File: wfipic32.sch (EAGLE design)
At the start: 31 parts, among them IC1 BMA490L, J1 MLE-105-01-G-DV, J2 MLE-105-01-G-DV, J3 MLE-105-01-G-DV, J4 MLE-105-01-G-DV, U1 PIC32MK0512MCJ048T-I/Y8XTQFP4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, U2 MAX6126B30

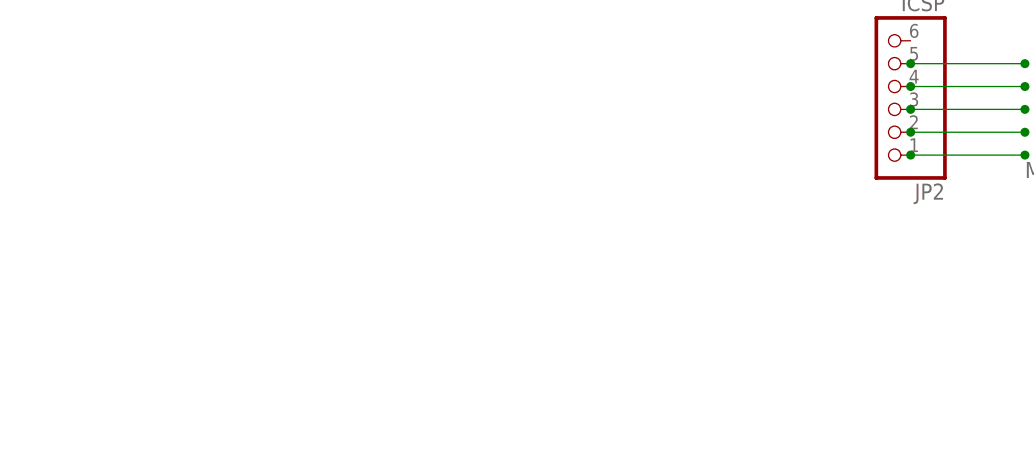
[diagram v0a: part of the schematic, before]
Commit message: up
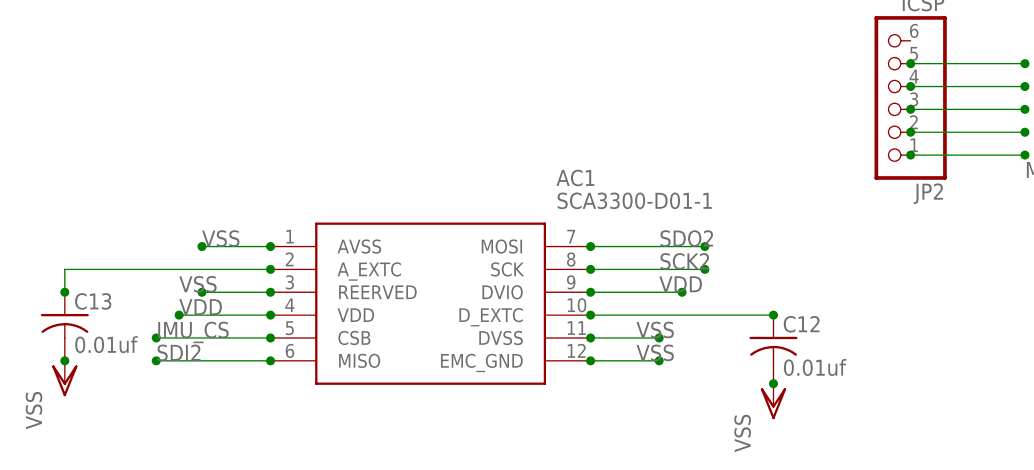
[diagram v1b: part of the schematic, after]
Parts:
- added AC1: SCA3300-D01-1, SCA3300-D01-1:SCA3300-D01-1
- added C12, C13: 0.01uf, rcl:C-USC0805
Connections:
- new net N$7: AC1.D_EXTC, C12.1
- new net N$9: AC1.A_EXTC, C13.1
- net IMU_CS: now also AC1.CSB
- net SCK2: now also AC1.SCK
- net SDI2: now also AC1.MISO
- net SDO2: now also AC1.MOSI
- net VDD: now also AC1.DVIO, AC1.VDD
- net VSS: now also AC1.AVSS, AC1.DVSS, AC1.EMC_GND, AC1.REERVED, C12.2, C13.2
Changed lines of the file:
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@@
 <part name="J4" library="MLE-105-01-G-DV" deviceset="MLE-105-01-G-DV" device=""/>
 <part name="VSS9" library="supply1" library_urn="urn:adsk.eagle:library:371" deviceset="VSS" device=""/>
+<part name="AC1" library="SCA3300-D01-1" deviceset="SCA3300-D01-1" device=""/>
+<part name="C12" library="rcl" library_urn="urn:adsk.eagle:library:334" deviceset="C-US" device="C0805" package3d_urn="urn:adsk.eagle:package:23617/2" value="0.01uf"/>
+<part name="C13" library="rcl" library_urn="urn:adsk.eagle:library:334" deviceset="C-US" device="C0805" package3d_urn="urn:adsk.eagle:package:23617/2" value="0.01uf"/>
+<part name="VSS21" library="supply1" library_urn="urn:adsk.eagle:library:371" deviceset="VSS" device=""/>
+<part name="VSS22" library="supply1" library_urn="urn:adsk.eagle:library:371" deviceset="VSS" device=""/>
 </parts>
 <sheets>
@@
 <instance part="VSS9" gate="G$1" x="93.98" y="139.7" smashed="yes" rot="R270">
 <attribute name="VALUE" x="88.9" y="142.24" size="1.778" layer="96"/>
+</instance>
+<instance part="AC1" gate="G$1" x="-30.48" y="-22.86" smashed="yes">
+<attribute name="NAME" x="1.27" y="-15.24" size="1.778" layer="95" align="center-left"/>
+<attribute name="VALUE" x="1.27" y="-17.78" size="1.778" layer="96" align="center-left"/>
+</instance>
+<instance part="C12" gate="G$1" x="25.4" y="-33.02" smashed="yes">
+<attribute name="NAME" x="26.416" y="-32.385" size="1.778" layer="95"/>
+<attribute name="VALUE" x="26.416" y="-37.211" size="1.778" layer="96"/>
+</instance>
+<instance part="C13" gate="G$1" x="-53.34" y="-30.48" smashed="yes">
+<attribute name="NAME" x="-52.324" y="-29.845" size="1.778" layer="95"/>
+<attribute name="VALUE" x="-52.324" y="-34.671" size="1.778" layer="96"/>
+</instance>
+<instance part="VSS21" gate="G$1" x="25.4" y="-40.64" smashed="yes">
+<attribute name="VALUE" x="22.86" y="-45.72" size="1.778" layer="96" rot="R90"/>
+</instance>
+<instance part="VSS22" gate="G$1" x="-53.34" y="-38.1" smashed="yes">
+<attribute name="VALUE" x="-55.88" y="-43.18" size="1.778" layer="96" rot="R90"/>
 </instance>
 </instances>
@@
 <junction x="132.08" y="144.78"/>
 </segment>
+<segment>
+<wire x1="-30.48" y1="-30.48" x2="-40.64" y2="-30.48" width="0.1524" layer="91"/>
+<pinref part="AC1" gate="G$1" pin="VDD"/>
+<label x="-40.64" y="-30.48" size="1.778" layer="95"/>
+<junction x="-30.48" y="-30.48"/>
+<junction x="-40.64" y="-30.48"/>
+</segment>
+<segment>
+<wire x1="15.24" y1="-27.94" x2="5.08" y2="-27.94" width="0.1524" layer="91"/>
+<pinref part="AC1" gate="G$1" pin="DVIO"/>
+<label x="12.7" y="-27.94" size="1.778" layer="95"/>
+<junction x="5.08" y="-27.94"/>
+<junction x="15.24" y="-27.94"/>
+</segment>
 </net>
 <net name="VSS" class="0">
@@
 <junction x="96.52" y="139.7"/>
 </segment>
+<segment>
+<wire x1="-30.48" y1="-22.86" x2="-38.1" y2="-22.86" width="0.1524" layer="91"/>
+<pinref part="AC1" gate="G$1" pin="AVSS"/>
+<label x="-38.1" y="-22.86" size="1.778" layer="95"/>
+<junction x="-30.48" y="-22.86"/>
+<junction x="-38.1" y="-22.86"/>
+</segment>
+<segment>
+<wire x1="12.7" y1="-33.02" x2="5.08" y2="-33.02" width="0.1524" layer="91"/>
+<pinref part="AC1" gate="G$1" pin="DVSS"/>
+<label x="10.16" y="-33.02" size="1.778" layer="95"/>
+<junction x="5.08" y="-33.02"/>
+<junction x="12.7" y="-33.02"/>
+</segment>
+<segment>
+<wire x1="12.7" y1="-35.56" x2="5.08" y2="-35.56" width="0.1524" layer="91"/>
+<pinref part="AC1" gate="G$1" pin="EMC_GND"/>
+<label x="10.16" y="-35.56" size="1.778" layer="95"/>
+<junction x="5.08" y="-35.56"/>
+<junction x="12.7" y="-35.56"/>
+</segment>
+<segment>
+<pinref part="C12" gate="G$1" pin="2"/>
+<pinref part="VSS21" gate="G$1" pin="VSS"/>
+<junction x="25.4" y="-38.1"/>
+</segment>
+<segment>
+<pinref part="C13" gate="G$1" pin="2"/>
+<pinref part="VSS22" gate="G$1" pin="VSS"/>
+<junction x="-53.34" y="-35.56"/>
+</segment>
+<segment>
+<wire x1="-30.48" y1="-27.94" x2="-38.1" y2="-27.94" width="0.1524" layer="91"/>
+<pinref part="AC1" gate="G$1" pin="REERVED"/>
+<label x="-40.64" y="-27.94" size="1.778" layer="95"/>
+<junction x="-38.1" y="-27.94"/>
+<junction x="-30.48" y="-27.94"/>
+</segment>
 </net>
 <net name="AVDD" class="0">
@@
 <junction x="132.08" y="147.32"/>
 </segment>
+<segment>
+<wire x1="-43.18" y1="-33.02" x2="-30.48" y2="-33.02" width="0.1524" layer="91"/>
+<pinref part="AC1" gate="G$1" pin="CSB"/>
+<label x="-43.18" y="-33.02" size="1.778" layer="95"/>
+<junction x="-30.48" y="-33.02"/>
+<junction x="-43.18" y="-33.02"/>
+</segment>
 </net>
 <net name="N$3" class="0">
@@
 <junction x="154.94" y="147.32"/>
 </segment>
+<segment>
+<wire x1="5.08" y1="-25.4" x2="17.78" y2="-25.4" width="0.1524" layer="91"/>
+<pinref part="AC1" gate="G$1" pin="SCK"/>
+<label x="12.7" y="-25.4" size="1.778" layer="95"/>
+<junction x="5.08" y="-25.4"/>
+<junction x="17.78" y="-25.4"/>
+</segment>
 </net>
 <net name="SDO2" class="0">
@@
 <junction x="154.94" y="137.16"/>
 </segment>
+<segment>
+<wire x1="17.78" y1="-22.86" x2="5.08" y2="-22.86" width="0.1524" layer="91"/>
+<pinref part="AC1" gate="G$1" pin="MOSI"/>
+<label x="12.7" y="-22.86" size="1.778" layer="95"/>
+<junction x="5.08" y="-22.86"/>
+<junction x="17.78" y="-22.86"/>
+</segment>
 </net>
 <net name="SDI2" class="0">
@@
 <label x="121.92" y="137.16" size="1.778" layer="95"/>
 <junction x="132.08" y="137.16"/>
+</segment>
+<segment>
+<wire x1="-43.18" y1="-35.56" x2="-30.48" y2="-35.56" width="0.1524" layer="91"/>
+<pinref part="AC1" gate="G$1" pin="MISO"/>
+<label x="-43.18" y="-35.56" size="1.778" layer="95"/>
+<junction x="-30.48" y="-35.56"/>
+<junction x="-43.18" y="-35.56"/>
 </segment>
 </net>
@@
 </segment>
 </net>
+<net name="N$7" class="0">
+<segment>
+<pinref part="AC1" gate="G$1" pin="D_EXTC"/>
+<wire x1="5.08" y1="-30.48" x2="25.4" y2="-30.48" width="0.1524" layer="91"/>
+<pinref part="C12" gate="G$1" pin="1"/>
+<junction x="5.08" y="-30.48"/>
+<junction x="25.4" y="-30.48"/>
+</segment>
+</net>
+<net name="N$9" class="0">
+<segment>
+<pinref part="AC1" gate="G$1" pin="A_EXTC"/>
+<pinref part="C13" gate="G$1" pin="1"/>
+<wire x1="-30.48" y1="-25.4" x2="-53.34" y2="-25.4" width="0.1524" layer="91"/>
+<wire x1="-53.34" y1="-25.4" x2="-53.34" y2="-27.94" width="0.1524" layer="91"/>
+<junction x="-53.34" y="-27.94"/>
+<junction x="-30.48" y="-25.4"/>
+</segment>
+</net>

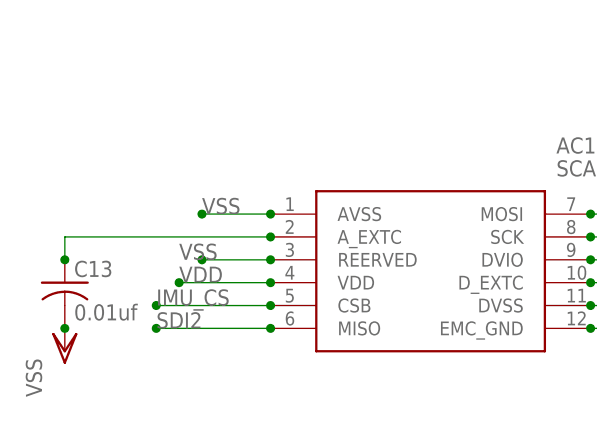
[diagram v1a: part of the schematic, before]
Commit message: up
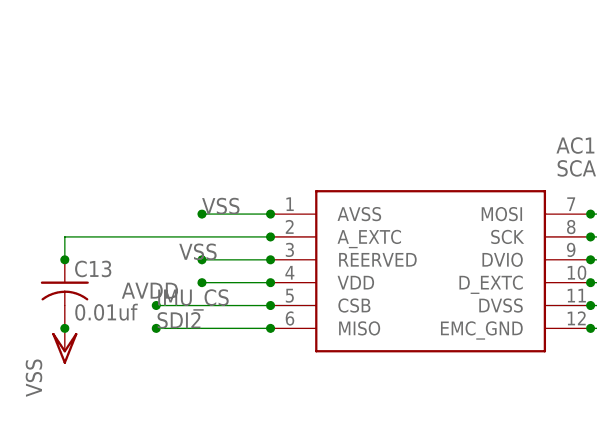
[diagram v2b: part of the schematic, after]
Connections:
- net AVDD: now also AC1.VDD
- net VDD: no longer AC1.VDD
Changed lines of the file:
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@@
-</segment>
-<segment>
-<wire x1="-30.48" y1="-30.48" x2="-40.64" y2="-30.48" width="0.1524" layer="91"/>
-<pinref part="AC1" gate="G$1" pin="VDD"/>
-<label x="-40.64" y="-30.48" size="1.778" layer="95"/>
-<junction x="-30.48" y="-30.48"/>
-<junction x="-40.64" y="-30.48"/>
 </segment>
 <segment>
@@
 <label x="76.2" y="0" size="1.778" layer="95"/>
 </segment>
+<segment>
+<wire x1="-30.48" y1="-30.48" x2="-38.1" y2="-30.48" width="0.1524" layer="91"/>
+<pinref part="AC1" gate="G$1" pin="VDD"/>
+<label x="-40.64" y="-30.48" size="1.778" layer="95" rot="R180"/>
+<junction x="-30.48" y="-30.48"/>
+<junction x="-38.1" y="-30.48"/>
+</segment>
 </net>
